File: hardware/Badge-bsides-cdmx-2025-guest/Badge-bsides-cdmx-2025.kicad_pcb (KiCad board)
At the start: 2 copper layers, 50.1 x 110 mm, 42 parts, among them J1 SWDIO, J3 ADDON, J4 Conn_01x04_Pin, J5 I2C, J6 Conn_01x04_Pin, P6 USB_C_Plug_USB2.0, Q3 DMG3415U-7, SW10 SW_Push, SW11 ON, SW2 RESET, SW7 SW_Push, SW8 SW_Push, SW9 SW_Push, U1 PY32F030F28U6TR, U6 AP2112K-3.3

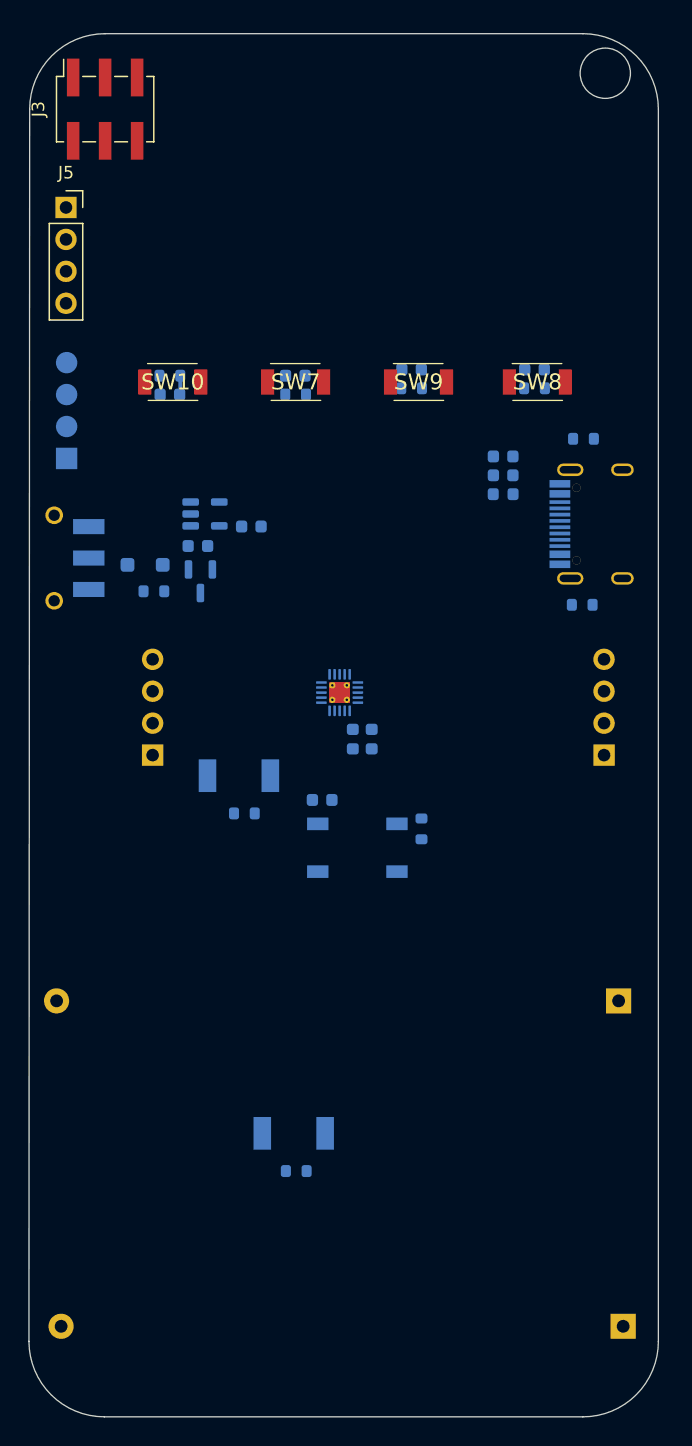
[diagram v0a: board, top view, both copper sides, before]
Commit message: Auto stash before merge of "main" and "origin/main"
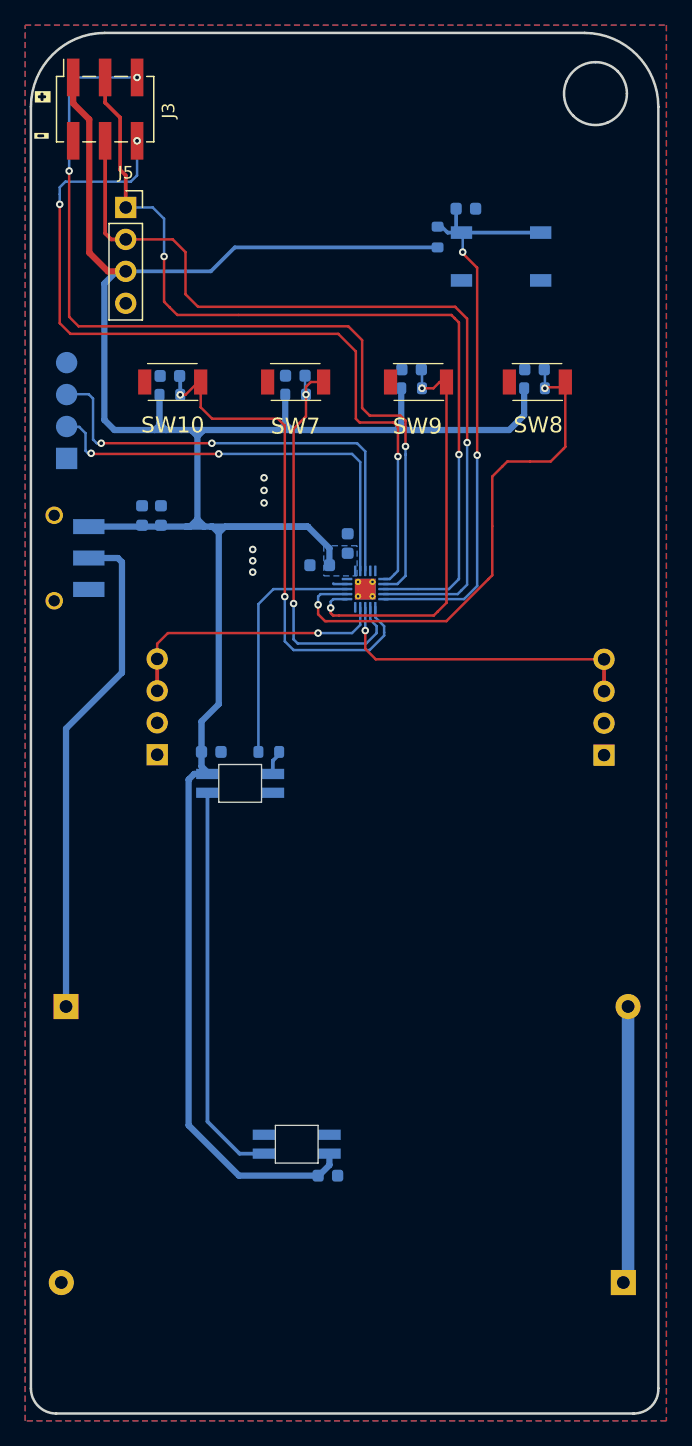
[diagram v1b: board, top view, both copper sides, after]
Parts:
- removed C10, C27: 10uF, Capacitor_SMD:C_0603_1608Metric
- removed D10, D9: R_LED, Footprints:LYT77K-K2M1
- removed D4: MBR120, Diode_SMD:D_SOD-123F
- removed F3: 750mA, Fuse:Fuse_0603_1608Metric
- removed P6: USB_C_Plug_USB2.0, Footprints:C393939
- removed Q3: DMG3415U-7, Package_TO_SOT_SMD:SOT-23
- removed R10: 100K, Resistor_SMD:R_0603_1608Metric
- removed R11, R9: 220, Resistor_SMD:R_0603_1608Metric
- removed R41, R45: 5k1, Resistor_SMD:R_0603_1608Metric
- removed U6: AP2112K-3.3, Package_TO_SOT_SMD:SOT-23-5
- added C31: 100nF, Capacitor_SMD:C_0603_1608Metric, B.Cu at (127.8, 95.8)
- added C32: 100nF, Capacitor_SMD:C_0603_1608Metric, B.Cu at (137.1, 129.5)
- added D21: SK6812MINI-E, Footprints:LED_SK6812-E, B.Cu at (130.1, 98.3)
- added D22: SK6812MINI-E, Footprints:LED_SK6812-E, B.Cu at (134.6, 127.0)
- added R12: 1K, Resistor_SMD:R_0603_1608Metric, B.Cu at (132.4, 95.8)
- added kibuzzard-684312AE: G***, kibuzzard-684312AE, B.Cu at (115.3, 74.8)
- added kibuzzard-684312C0: G***, kibuzzard-684312C0, B.Cu at (115.4, 85.9)
- added kibuzzard-684312D7: G***, kibuzzard-684312D7, B.Cu at (151.1, 60.3)
- added kibuzzard-684312EA: G***, kibuzzard-684312EA, F.Cu at (114.4, 43.7)
- added kibuzzard-684312F6: G***, kibuzzard-684312F6, F.Cu at (114.3, 46.8)
- added kibuzzard-68431305: G***, kibuzzard-68431305, B.Cu at (116.9, 57.5)
- added kibuzzard-6843130E: G***, kibuzzard-6843130E, B.Cu at (117.0, 60.3)
- moved C6 48.4 mm to (148.1, 52.6)
- moved SW2 48.4 mm to (150.8, 56.4)
- moved R4 47.1 mm to (145.8, 54.9)
- moved BT3 44.0 mm to (116.2, 116.0), turned to 0 degrees
- moved C33 27.6 mm to (123.8, 77.0), turned to 90 degrees
- moved C34 15.6 mm to (138.7, 79.2), turned to 90 degrees
- moved C28 14.4 mm to (136.4, 81.0), turned to 180 degrees
- moved C26 8.73 mm to (122.3, 77.0), turned to 90 degrees
- moved U1 8.48 mm to (140.1, 82.8), turned to 0 degrees
- moved J5 4.75 mm to (121.0, 52.5)
- moved BT4 3.48 mm to (160.6, 138.0)
- moved R8 1.52 mm to (124.5, 67.4)
- moved C70 1.48 mm to (124.5, 65.9)
- moved J6 0.36 mm to (123.5, 96.0)
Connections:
- BT3 pad 1: Net-(BT3--) -> +BATT
- BT3 pad 2: +BATT -> Net-(BT3--)
- BT4 pad 1: GND -> Net-(BT3--)
- BT4 pad 2: Net-(BT3--) -> GND
- C26 pad 1: +3V3 -> +3.3V
- C33 pad 1: VBUS -> +3.3V
- J3 pad 1: +3V3 -> +3.3V
- J4 pad 3: /RX -> /TX
- J4 pad 4: /RX -> /TX
- J6 pad 3: /TX -> /RX
- J6 pad 4: /TX -> /RX
- R4 pad 2: +3V3 -> +3.3V
- R5 pad 2: +3V3 -> +3.3V
- R6 pad 2: +3V3 -> +3.3V
- R7 pad 2: +3V3 -> +3.3V
- R8 pad 2: +3V3 -> +3.3V
- SW11 pad 2: Net-(D4-K) -> +BATT
- SW11 pad 3: Net-(SW11-A) -> +3.3V
- U1 pad 10: /LED1 -> unconnected-(U1-PB6-Pad10)
- U1 pad 11: unconnected-(U1-PB7-Pad11) -> /GPIO1
- U1 pad 12: unconnected-(U1-PF4/BOOT0-Pad12) -> /GPIO2
- U1 pad 20: /LED2 -> unconnected-(U1-PA4-Pad20)
- U1 pad 3: /GPIO1 -> /NEO
- U1 pad 5: /GPIO2 -> unconnected-(U1-PA12-Pad5)
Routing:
- net +3.3V: track 0.07 -> 206.7 mm
- net /GPIO2: track 0.00 -> 71.9 mm, vias 0 -> 3
- net /SDA: track 0.00 -> 71.9 mm, vias 0 -> 2
- net /SCL: track 0.03 -> 69.0 mm, vias 0 -> 1
- net /GPIO1: track 0.00 -> 66.4 mm, vias 0 -> 3
- net /NTST: track 0.00 -> 47.0 mm, vias 0 -> 2
- net /BTTN1: track 0.00 -> 42.5 mm, vias 0 -> 2
- net +BATT: track 0.00 -> 40.0 mm
- net /BTTN4: track 1.52 -> 41.2 mm, vias 0 -> 2
- net /SWCLK: track 0.00 -> 37.1 mm, vias 0 -> 2
- net /SWDIO: track 0.00 -> 34.0 mm, vias 0 -> 2
- net /BTTN2: track 0.00 -> 33.2 mm, vias 0 -> 2
- net /BTTN3: track 0.00 -> 32.9 mm, vias 0 -> 2
- net Net-(D21-DOUT): track 0.00 -> 31.7 mm
- net /TX: track 0.00 -> 25.2 mm, vias 0 -> 1
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- added copper zone on B.Cu, net +3.3V
- added copper zone on B.Cu, net GND
- added copper zone on F.Cu, net GND
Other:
- board size 50.1 x 110 mm -> 49.9 x 109.8 mm
